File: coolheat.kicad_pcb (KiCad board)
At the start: 2 copper layers, 73.7 x 73.7 mm, 16 parts, among them J1 Screw_Terminal_01x02, J2 Screw_Terminal_01x03, J3 Screw_Terminal_01x03, J4 Screw_Terminal_01x03, J5 Screw_Terminal_01x02, J6 Screw_Terminal_01x02, J7 Screw_Terminal_01x02, J8 Screw_Terminal_01x02, K1 Finder 41.31.8.230.0000, K2 Finder 41.31.8.230.0000, K3 Finder 41.31.8.230.0000, K4 Finder 41.31.8.230.0000

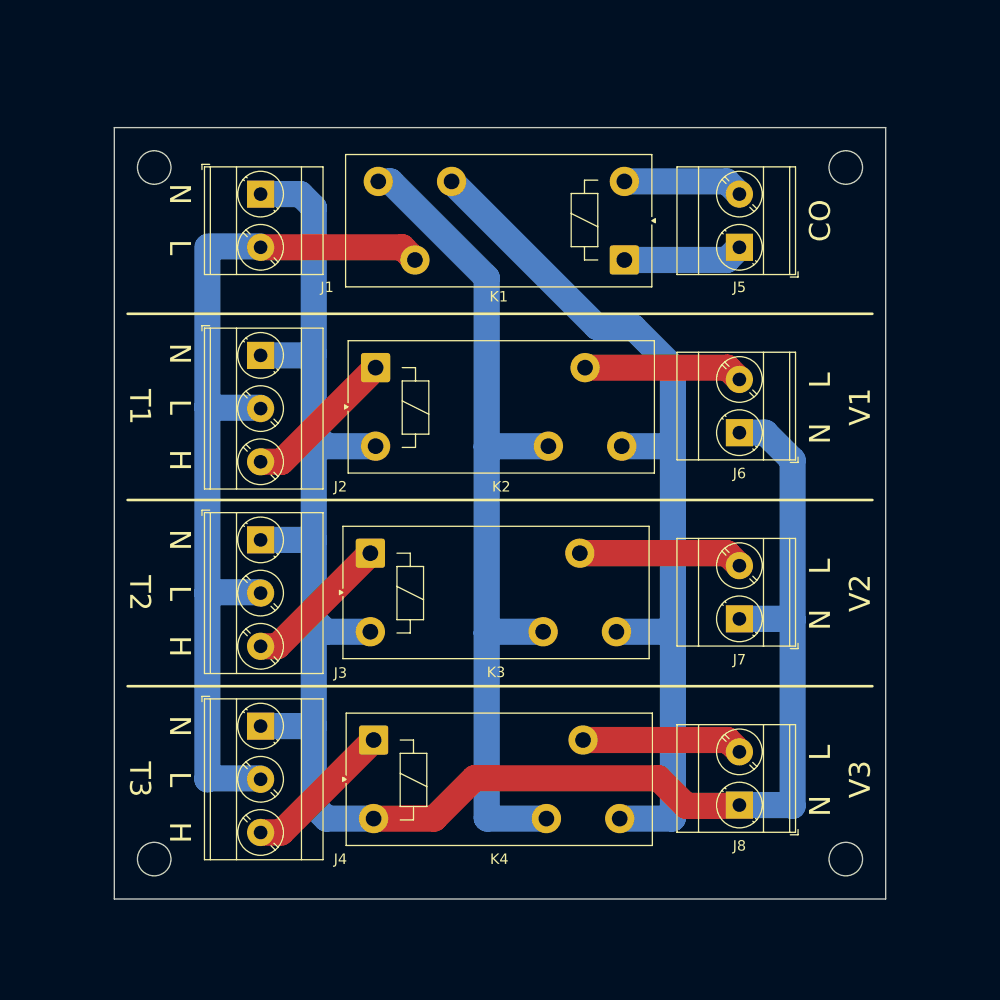
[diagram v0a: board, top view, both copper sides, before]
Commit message: hensel case
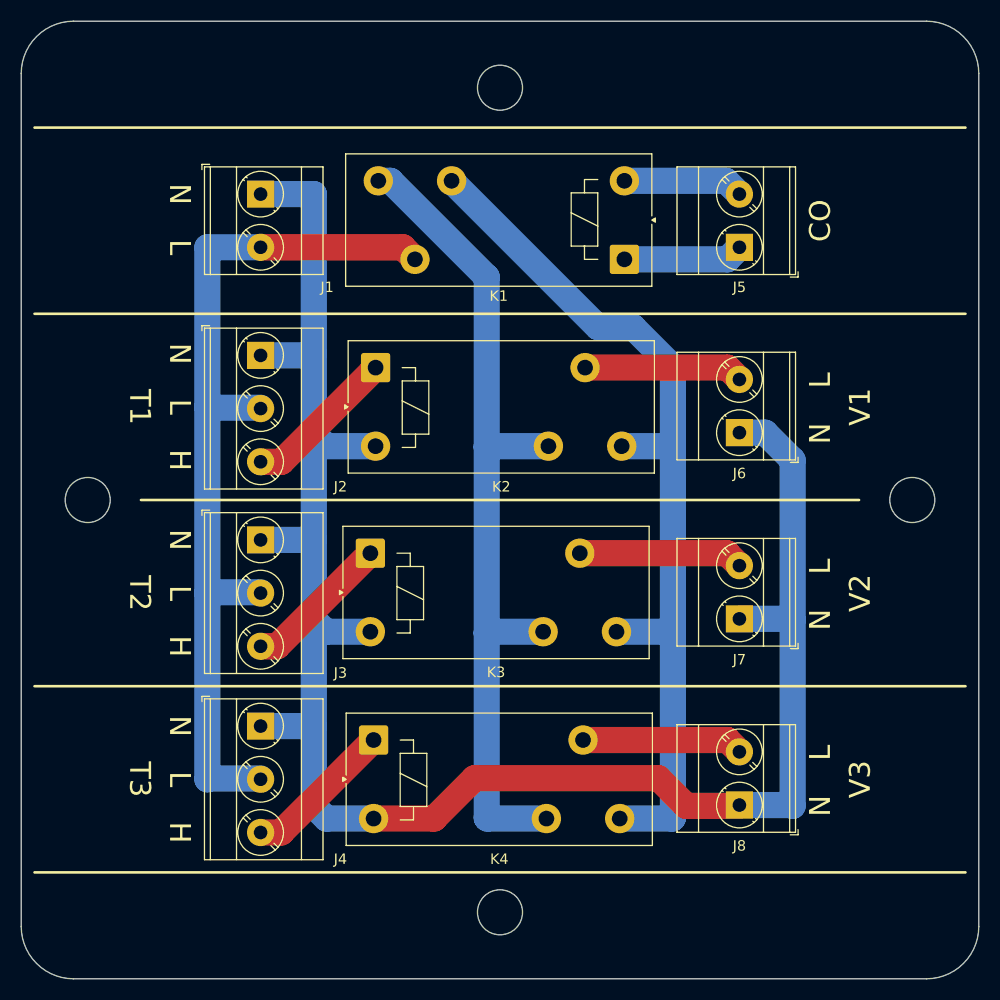
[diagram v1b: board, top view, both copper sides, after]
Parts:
- H1, H2, H3, H4: footprint MountingHole:MountingHole_3.2mm_M3 -> MountingHole:MountingHole_4.3mm_M4
- J1: value Screw_Terminal_01x02 -> SUPPLY
- J2: value Screw_Terminal_01x03 -> THERMOSTAT 1
- J3: value Screw_Terminal_01x03 -> THERMOSTAT 2
- J4: value Screw_Terminal_01x03 -> THERMOSTAT 3
- J5: value Screw_Terminal_01x02 -> CHAGEOVER
- J6: value Screw_Terminal_01x02 -> VALVE 1
- J7: value Screw_Terminal_01x02 -> VALVE 2
- J8: value Screw_Terminal_01x02 -> VALVE 3
- moved H3 80.1 mm to (148.6, 110.5)
- moved H4 33.9 mm to (109.2, 71.1)
- moved H1 33.4 mm to (109.2, 149.9)
- moved H2 32.4 mm to (69.8, 110.5)
- moved K1 0.06 mm to (121.1, 87.5)
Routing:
- net Net-(J1-Pin_1): track 183.6 -> 184.4 mm
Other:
- board size 73.7 x 73.7 mm -> 91.4 x 91.4 mm

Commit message: almost done
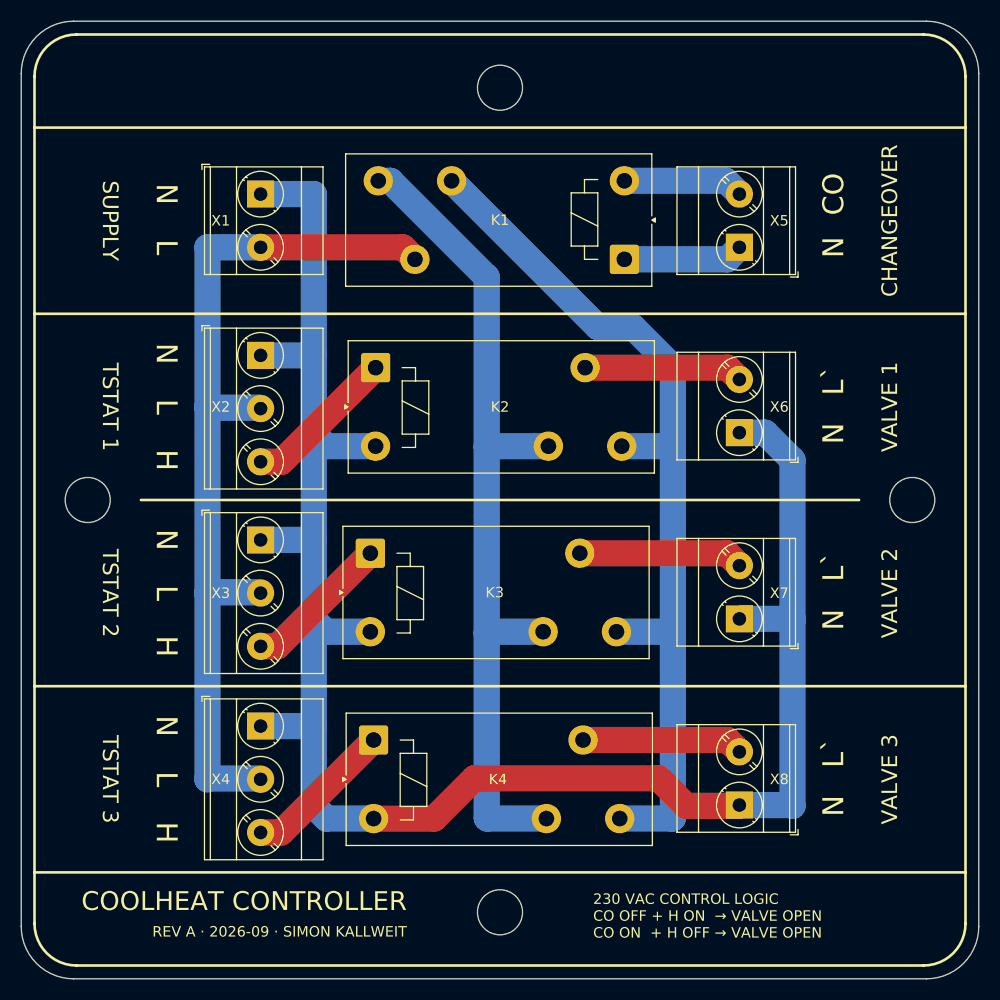
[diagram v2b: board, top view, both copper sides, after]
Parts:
- X5: renamed from J5; value CHAGEOVER -> CHANGEOVER
- renumbered J1 to X1, J2 to X2, J3 to X3, J4 to X4, J6 to X6, J7 to X7, J8 to X8
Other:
- board text added: "230 VAC CONTROL LOGIC CO OFF + H ON → VALVE OPEN CO ON + H OFF → VALVE OPEN"
- board text added: "CHANGEOVER"
- board text added: "COOLHEAT CONTROLLER"
- board text added: "L`"
- board text added: "REV A · 2026-09 · SIMON KALLWEIT"
- board text added: "SUPPLY"
- board text added: "TSTAT 1"
- board text added: "TSTAT 2"
- board text added: "TSTAT 3"
- board text added: "VALVE 1"
- board text added: "VALVE 2"
- board text added: "VALVE 3"
- board text removed: "T1"
- board text removed: "T2"
- board text removed: "T3"
- board text removed: "V1"
- board text removed: "V2"
- board text removed: "V3"

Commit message: production design
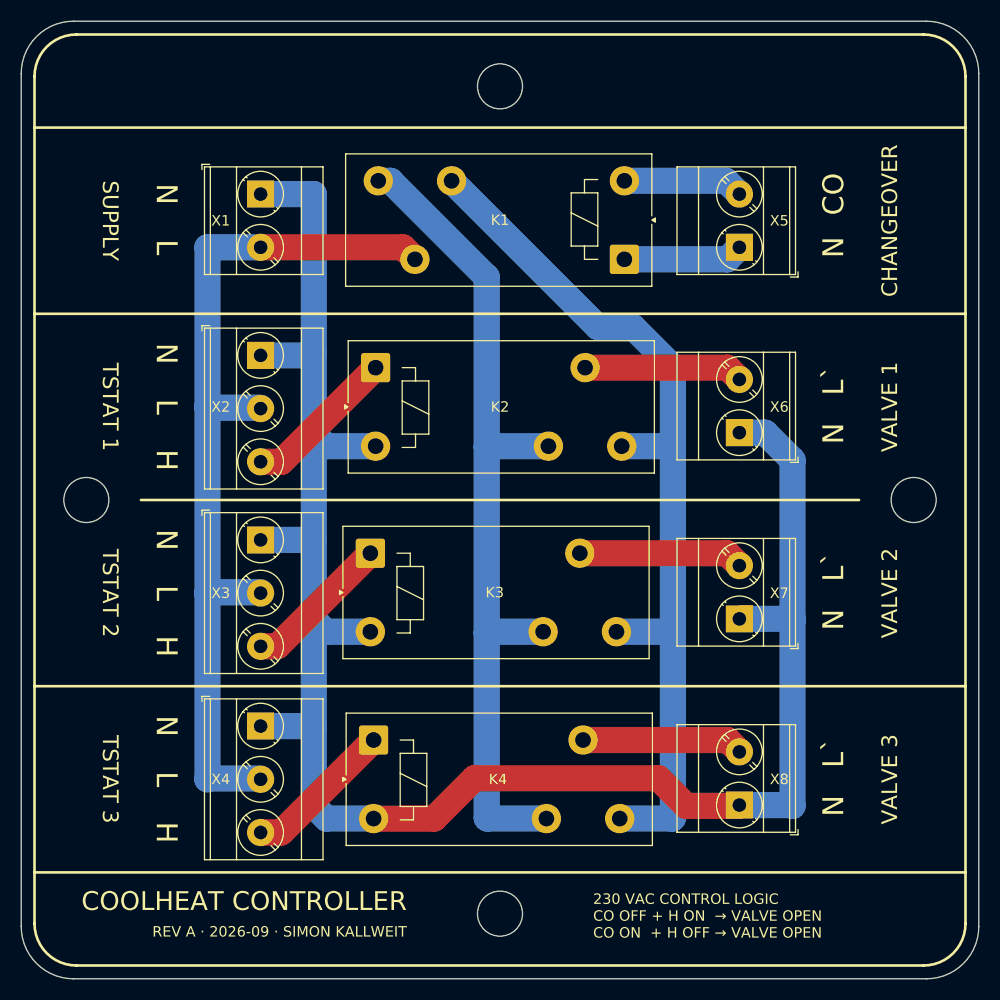
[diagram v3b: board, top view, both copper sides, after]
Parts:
- moved H4 0.13 mm to (109.2, 71.0)
- moved H1 0.13 mm to (109.2, 150.0)
- moved H2 0.13 mm to (69.7, 110.5)
- moved H3 0.13 mm to (148.7, 110.5)
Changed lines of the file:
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@@
 		(pad_to_mask_clearance 0)
 		(allow_soldermask_bridges_in_footprints no)
-		(grid_origin 72.39 74.93)
+		(grid_origin 109.22 110.49)
 		(pcbplotparams
 			(layerselection 0x00010fc_ffffffff)
@@
 	(footprint "MountingHole:MountingHole_4.3mm_M4"
 		(layer "F.Cu")
-		(at 109.22 149.86)
+		(at 109.22 149.99)
 		(descr "Mounting Hole 4.3mm, no annular, M4")
 		(tags "mounting hole 4.3mm no annular m4")
@@
 	(footprint "MountingHole:MountingHole_4.3mm_M4"
 		(layer "F.Cu")
-		(at 69.85 110.49)
+		(at 69.72 110.49)
 		(descr "Mounting Hole 4.3mm, no annular, M4")
 		(tags "mounting hole 4.3mm no annular m4")
@@
 	(footprint "MountingHole:MountingHole_4.3mm_M4"
 		(layer "F.Cu")
-		(at 109.22 71.12)
+		(at 109.22 70.99)
 		(descr "Mounting Hole 4.3mm, no annular, M4")
 		(tags "mounting hole 4.3mm no annular m4")
@@
 	(footprint "MountingHole:MountingHole_4.3mm_M4"
 		(layer "F.Cu")
-		(at 148.59 110.49)
+		(at 148.72 110.49)
 		(descr "Mounting Hole 4.3mm, no annular, M4")
 		(tags "mounting hole 4.3mm no annular m4")
